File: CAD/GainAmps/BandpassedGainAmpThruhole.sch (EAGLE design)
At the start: 9 parts, among them U1 OPA202IDR

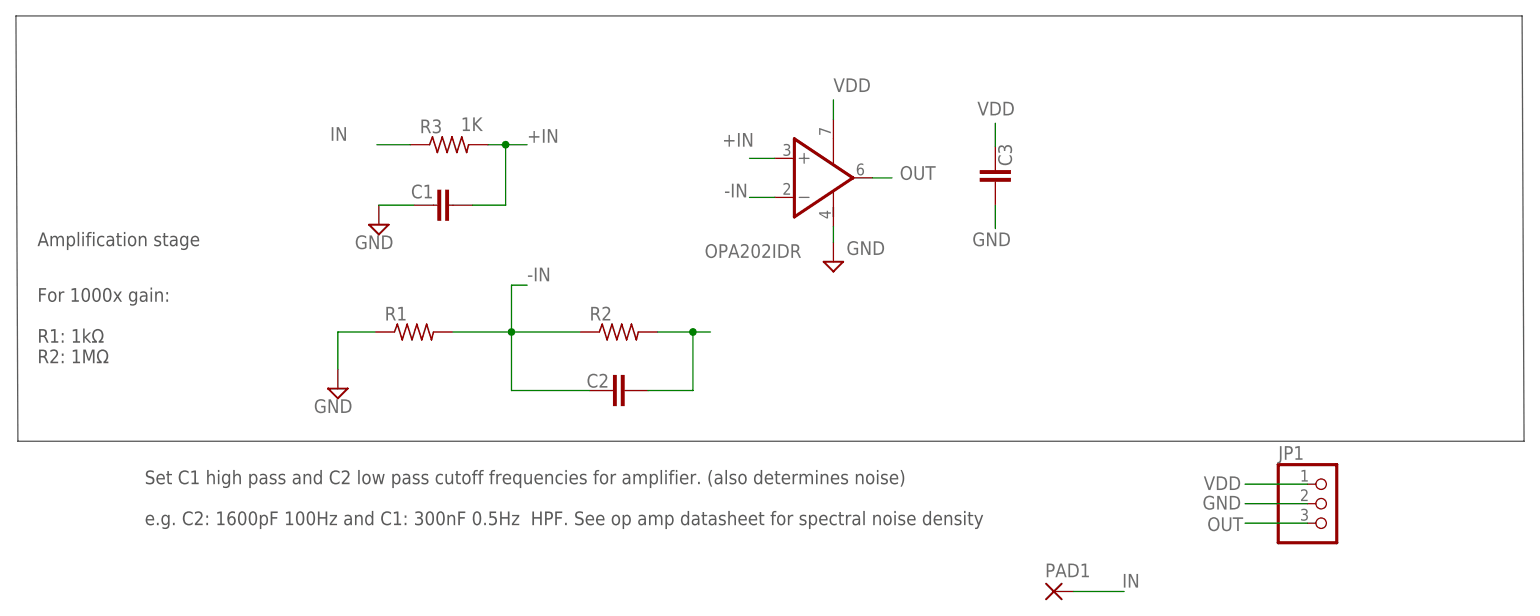
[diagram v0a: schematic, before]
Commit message: fixes
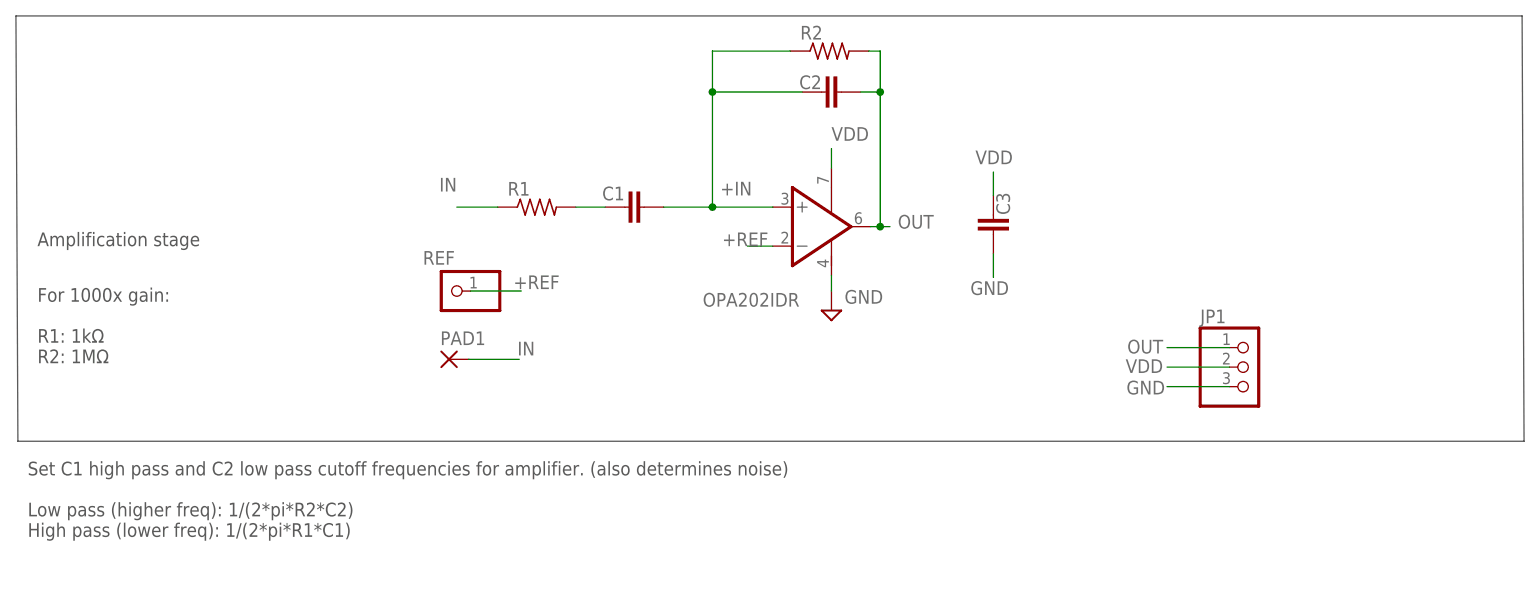
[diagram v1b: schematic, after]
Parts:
- removed R3: 1K, rcl:R-US_0204/5
- added REF: (no value), pinhead:PINHD-1X1
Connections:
- removed net -IN: C2.1, R1.2, R2.1, U1A.-IN
- removed net N$3: C2.2, R2.2
- new net +REF: REF.1, U1A.-IN
- new net R1C1: C1.1, R1.2
- net +IN: now also C2.1, R2.1; no longer R3.2
- net GND: now also JP1.3; no longer C1.1, JP1.2, R1.1
- net IN: now also R1.1; no longer R3.1
- net OUT: now also C2.2, JP1.1, R2.2; no longer JP1.3
- net VDD: now also JP1.2; no longer JP1.1
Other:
- note added: "Set C1 high pass and C2 low pass cutoff frequencies for amplifier. (also determines noise) Low pass (higher freq): 1/(2*pi*R2*C2) High pass (lower freq): 1/(2*pi*R1*C1)"
- note removed: "Set C1 high pass and C2 low pass cutoff frequencies for amplifier. (also determines noise) e.g. C2: 1600pF 100Hz and C1: 300nF 0.5Hz HPF. See op amp datasheet for spectral noise density"
- moved on the sheet: C1, C2, C3, JP1, PAD1, R1, R2
